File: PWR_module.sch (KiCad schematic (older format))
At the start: 4 parts

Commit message: updated links
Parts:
- PWR_AC/DC_+!2V1: alternative cheap (none) -> http://hu.farnell.com/vigortronix/vtx-214-010-205/power-sup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
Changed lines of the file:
@@
 F 2 "water:VTX-214-015-112" H 5200 2650 60  0001 C CNN
 F 3 "http://hu.farnell.com/tdk-lambda/kms-15a-5/power-supply-ac-dc-5v-3a/dp/2664694" H 5200 2650 60  0001 C CNN
+F 4 "http://hu.farnell.com/vigortronix/vtx-214-010-205/power-supply-ac-dc-5v-2a/dp/2464685" H 5200 2650 60  0001 C CNN "alternative cheap"
 	1    5200 2650
 	1    0    0    -1

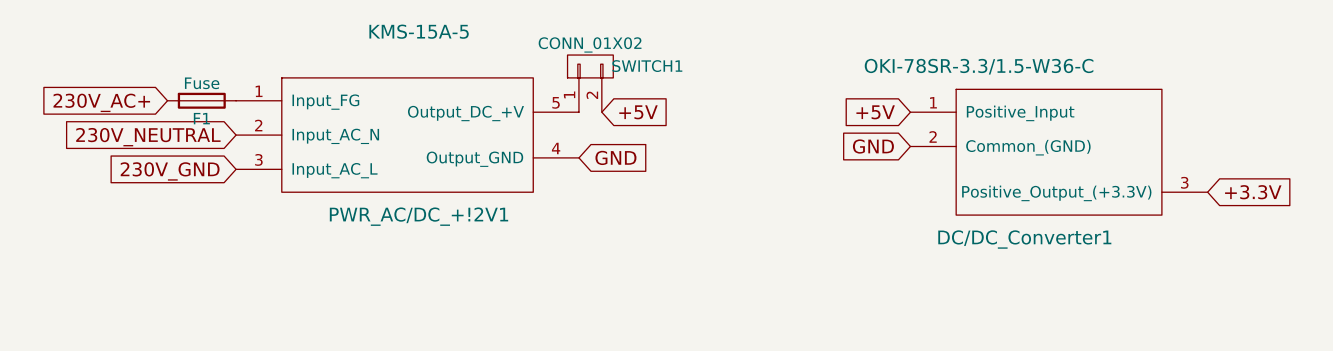
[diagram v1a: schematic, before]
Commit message: stash commit before the revision of the parts
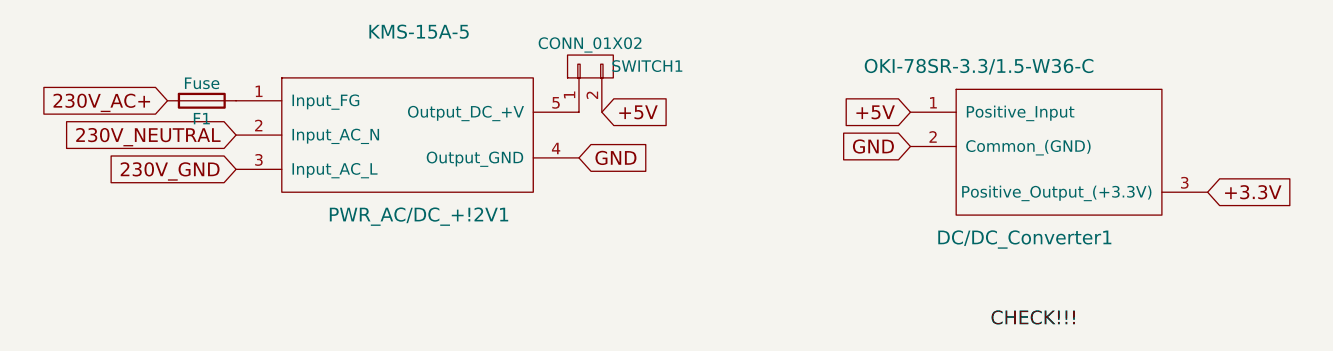
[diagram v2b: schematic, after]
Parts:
- DC/DC_Converter1: small power 0.5A (none) -> http://hu.farnell.com/texas-instruments/ua78m33qdcyrg4q1/li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
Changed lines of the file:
@@
 F 2 "water:OKI-78SR-3.3-1.5-W36-C" H 7650 2800 60  0001 C CNN
 F 3 "http://hu.farnell.com/murata-power-solutions/oki-78sr-3-3-1-5-w36-c/sr-dc-dc-converter-sip-module/dp/2102100" H 7650 2800 60  0001 C CNN
+F 4 "http://hu.farnell.com/texas-instruments/ua78m33qdcyrg4q1/linear-voltreg-3-3v-0-5a-sot-223/dp/2463957?ost=2463957&searchView=table&iscrfnonsku=false&ddkey=http%3Ahu-HU%2FElement14_Hungary%2Fsearch" H 7650 2800 60  0001 C CNN "small power 0.5A"
 	1    7650 2800
 	1    0    0    -1
@@
 	0    1    1    0
 $EndComp
+Text Label 7700 3950 0    60   ~ 0
+CHECK!!!
 $EndSCHEMATC
